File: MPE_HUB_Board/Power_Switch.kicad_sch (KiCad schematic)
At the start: 9 parts, among them U5 VND7050AJTR

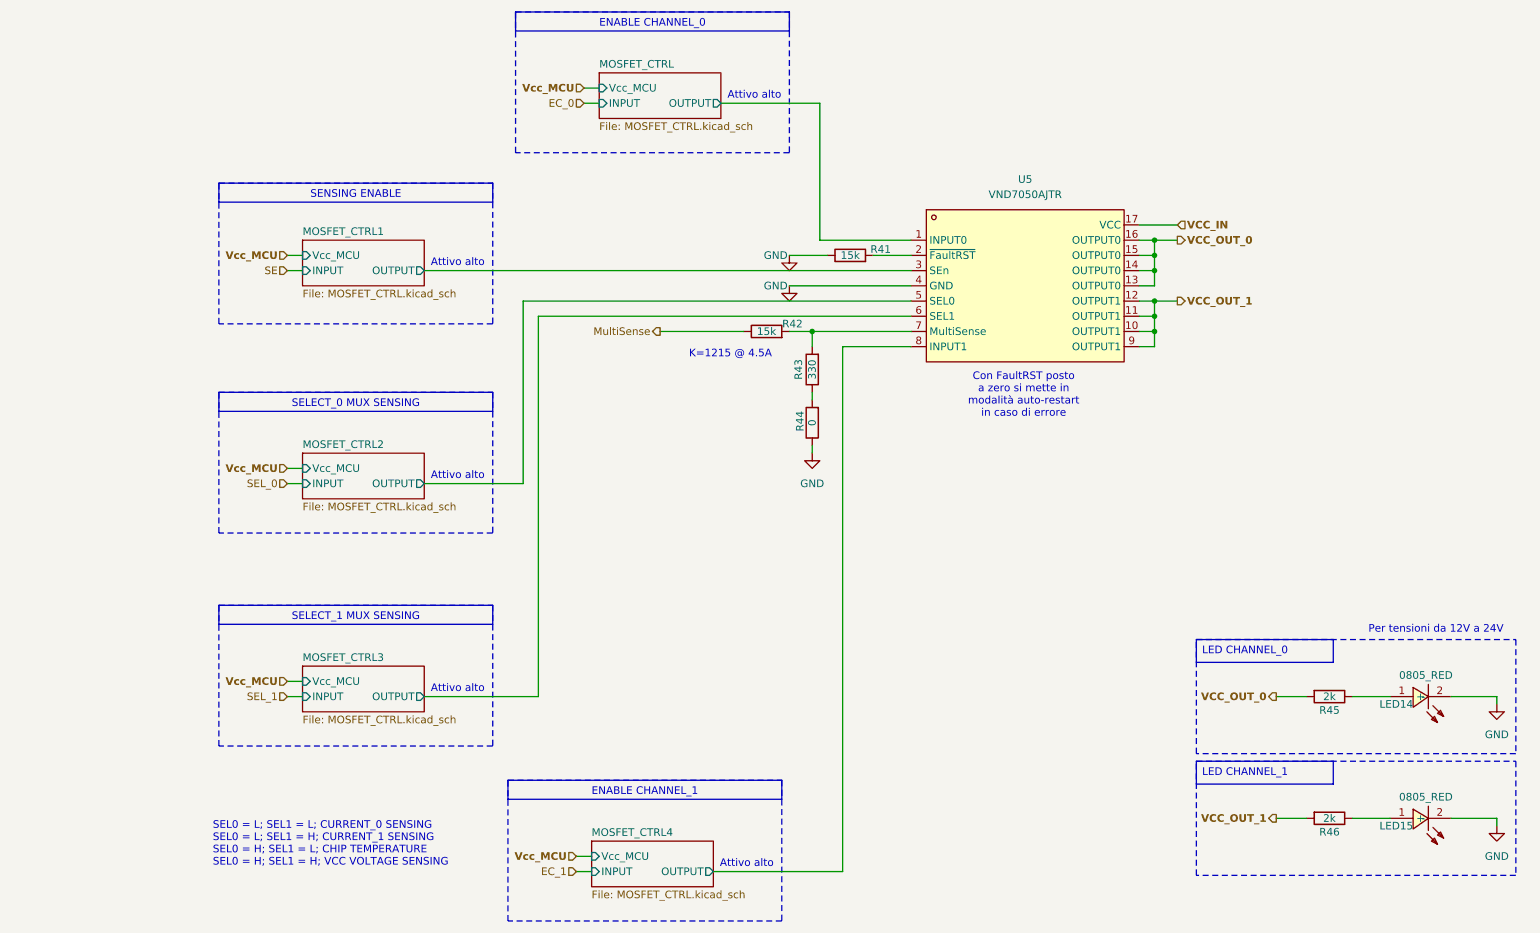
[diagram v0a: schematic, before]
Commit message: Update 04/07/2025
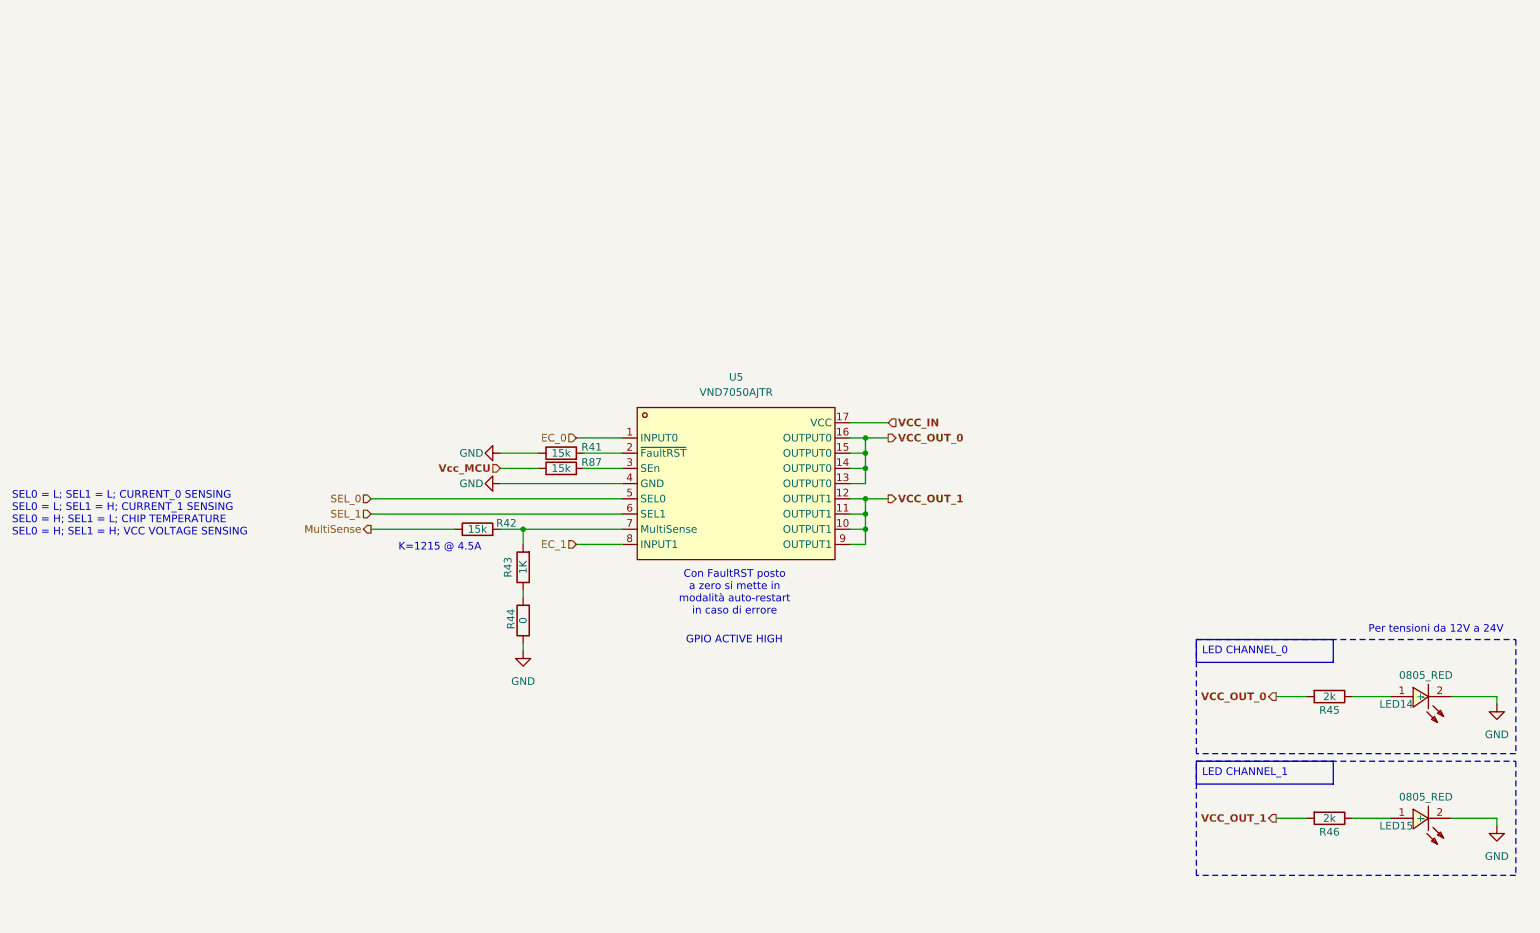
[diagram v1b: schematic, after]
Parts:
- added R87: 15k, Resistor_SMD:R_0603_1608Metric, symbol Device:R
- R43: value 330 -> 1K; LCSC C23138 -> C21190; LCSC Part (none) -> C21190
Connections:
- net MOSFET_CTRL/OUTPUT is gone; now on net EC_0: U5.1 (INPUT0)
- net MOSFET_CTRL2/OUTPUT is gone; now on net SEL_0: U5.5 (SEL0)
- net MOSFET_CTRL3/OUTPUT is gone; now on net SEL_1: U5.6 (SEL1)
- net MOSFET_CTRL4/OUTPUT is gone; now on net EC_1: U5.8 (INPUT1)
- net Vcc_MCU: now also R87.1
- net MOSFET_CTRL1/OUTPUT: no longer names the net of U5.3 (SEn)
- net MOSFET_CTRL1/OUTPUT: now also R87.2
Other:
- removed sheet MOSFET_CTRL
- removed sheet MOSFET_CTRL1
- removed sheet MOSFET_CTRL2
- removed sheet MOSFET_CTRL3
- removed sheet MOSFET_CTRL4
- note added: "GPIO ACTIVE HIGH"
- note removed: "Attivo alto"
- moved on the sheet: R41, R42, R44, U5

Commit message: Update 08/07/2025
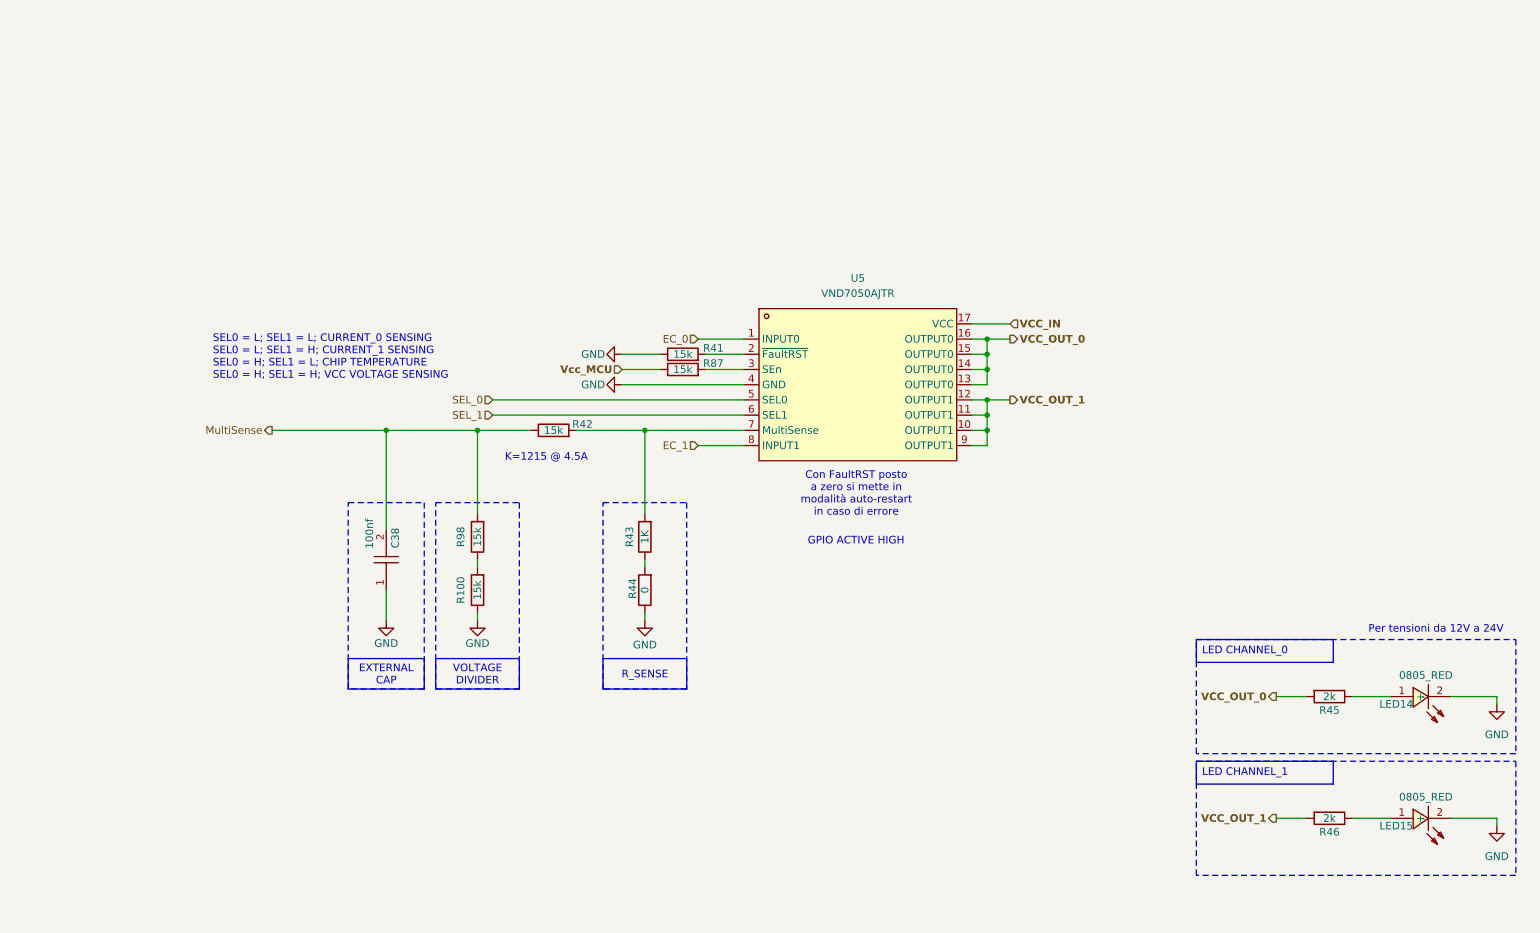
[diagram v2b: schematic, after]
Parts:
- added C38: 100nf, Capacitor_SMD:C_0603_1608Metric, symbol easyeda2kicad:CC0603KRX7R9BB104
- added R100, R98: 15k, Resistor_SMD:R_0603_1608Metric, symbol Device:R
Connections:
- net GND: now also C38.1, R100.1
- net MultiSense: now also C38.2, R98.2
- new net: R100.2, R98.1
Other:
- moved on the sheet: R41, R42, R43, R44, R87, U5

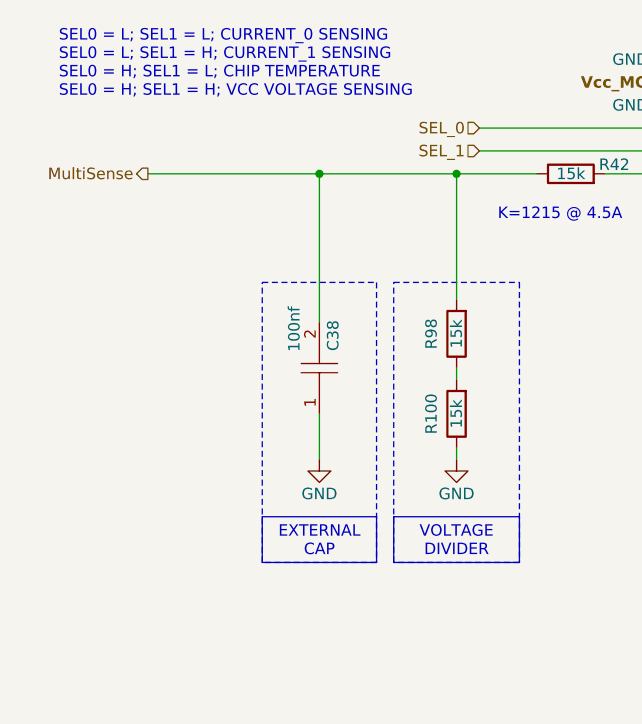
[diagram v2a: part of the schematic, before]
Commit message: HUB Hardware V1.1.0
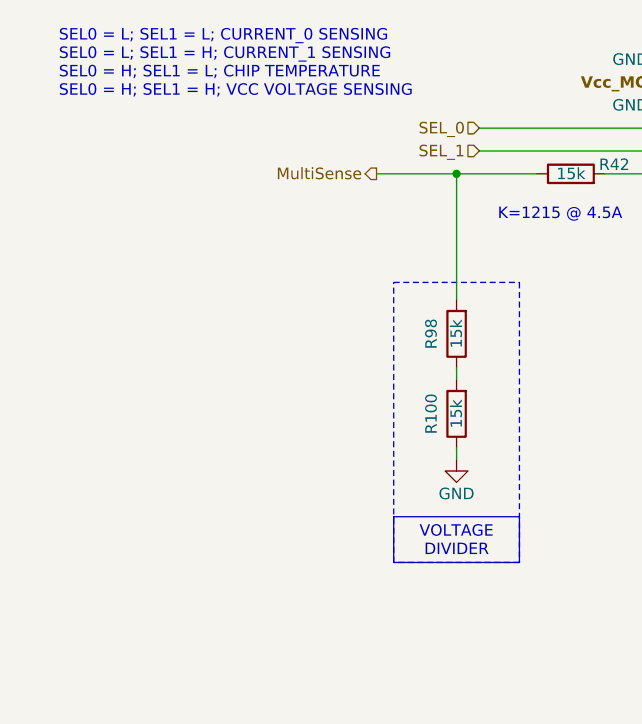
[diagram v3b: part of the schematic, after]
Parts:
- removed C38: 100nf, Capacitor_SMD:C_0603_1608Metric, symbol easyeda2kicad:CC0603KRX7R9BB104
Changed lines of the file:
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@@
-	)
-	(rectangle
-		(start 87.63 100.965)
-		(end 100.33 132.08)
-		(stroke
-			(width 0)
-			(type dot)
-			(color 0 132 0 1)
-		)
-		(fill
-			(type none)
-		)
 	)
 	(rectangle
@@
 		(at 102.235 127 0)
 		(size 13.97 5.08)
-		(margins 0.9525 0.9525 0.9525 0.9525)
-		(stroke
-			(width 0)
-			(type solid)
-			(color 0 132 0 1)
-		)
-		(fill
-			(type none)
-		)
-		(effects
-			(font
-				(size 1.27 1.27)
-				(color 0 132 0 1)
-			)
-		)
-	)
-	(text_box "EXTERNAL CAP"
-		(exclude_from_sim no)
-		(at 87.63 127 0)
-		(size 12.7 5.08)
 		(margins 0.9525 0.9525 0.9525 0.9525)
 		(stroke
@@
 	)
 	(junction
-		(at 93.98 88.9)
-		(diameter 0)
-		(color 0 0 0 0)
-	)
-	(junction
 		(at 194.31 78.74)
 		(diameter 0)
@@
 	(wire
 		(pts
-			(xy 93.98 115.57) (xy 93.98 120.65)
-		)
-		(stroke
-			(width 0)
-			(type default)
-		)
-	)
-	(wire
-		(pts
 			(xy 137.16 119.38) (xy 137.16 120.65)
 		)
@@
 	(wire
 		(pts
-			(xy 74.93 88.9) (xy 93.98 88.9)
-		)
-		(stroke
-			(width 0)
-			(type default)
-		)
-	)
-	(wire
-		(pts
-			(xy 93.98 88.9) (xy 93.98 105.41)
-		)
-		(stroke
-			(width 0)
-			(type default)
-		)
-	)
-	(wire
-		(pts
 			(xy 271.78 133.35) (xy 279.4 133.35)
 		)
@@
 	(wire
 		(pts
-			(xy 93.98 88.9) (xy 109.22 88.9)
+			(xy 100.33 88.9) (xy 109.22 88.9)
 		)
 		(stroke
@@
 	(hierarchical_label "MultiSense"
 		(shape output)
-		(at 74.93 88.9 180)
+		(at 100.33 88.9 180)
 		(effects
 			(font
@@
 				(path "/6490f62d-7c0a-4455-8633-837f094f0a1c/36a1afe1-9d7e-4453-8bd5-557c8a4303ef"
 					(reference "#PWR051")
-					(unit 1)
-				)
-			)
-		)
-	)
-	(symbol
-		(lib_name "CC0603KRX7R9BB104_2")
-		(lib_id "easyeda2kicad:CC0603KRX7R9BB104")
-		(at 93.98 110.49 90)
-		(unit 1)
-		(exclude_from_sim no)
-		(in_bom yes)
-		(on_board yes)
-		(dnp no)
-		(property "Reference" "C38"
-			(at 95.504 105.156 0)
-			(effects
-				(font
-					(size 1.27 1.27)
-				)
-				(justify right)
-			)
-		)
-		(property "Value" "100nf"
-			(at 91.186 103.632 0)
-			(effects
-				(font
-					(size 1.27 1.27)
-				)
-				(justify right)
-			)
-		)
-		(property "Footprint" "Capacitor_SMD:C_0603_1608Metric"
-			(at 101.6 110.49 0)
-			(effects
-				(font
-					(size 1.27 1.27)
-				)
-				(hide yes)
-			)
-		)
-		(property "Datasheet" "https://lcsc.com/product-detail/Multilayer-Ceramic-Capacitors-MLCC-SMD-SMT_100nF-104-10-50V_C14663.html"
-			(at 104.14 110.49 0)
-			(effects
-				(font
-					(size 1.27 1.27)
-				)
-				(hide yes)
-			)
-		)
-		(property "Description" ""
-			(at 93.98 110.49 0)
-			(effects
-				(font
-					(size 1.27 1.27)
-				)
-				(hide yes)
-			)
-		)
-		(property "LCSC Part" "C14663"
-			(at 106.68 110.49 0)
-			(effects
-				(font
-					(size 1.27 1.27)
-				)
-				(hide yes)
-			)
-		)
-		(property "LCSC" "C14663"
-			(at 95.885 107.95 0)
-			(effects
-				(font
-					(size 1.27 1.27)
-				)
-				(hide yes)
-			)
-		)
-		(pin "1"
-		)
-		(pin "2"
-		)
-		(instances
-			(project "HUB_MPE"
-				(path "/6490f62d-7c0a-4455-8633-837f094f0a1c/26b9dfe9-c957-43ca-ba2b-36e349e2ebb9"
-					(reference "C39")
-					(unit 1)
-				)
-				(path "/6490f62d-7c0a-4455-8633-837f094f0a1c/36a1afe1-9d7e-4453-8bd5-557c8a4303ef"
-					(reference "C38")
 					(unit 1)
 				)
@@
 					(unit 1)
 				)
-			)
-		)
-	)
-	(symbol
-		(lib_id "power:GND")
-		(at 93.98 120.65 0)
-		(unit 1)
-		(exclude_from_sim no)
-		(in_bom yes)
-		(on_board yes)
-		(dnp no)
-		(property "Reference" "#PWR083"
-			(at 93.98 127 0)
-			(effects
-				(font
-					(size 1.27 1.27)
-				)
-				(hide yes)
-			)
-		)
-		(property "Value" "GND"
-			(at 93.98 124.46 0)
-			(effects
-				(font
-					(size 1.27 1.27)
-				)
-			)
-		)
-		(property "Footprint" ""
-			(at 93.98 120.65 0)
-			(effects
-				(font
-					(size 1.27 1.27)
-				)
-				(hide yes)
-			)
-		)
-		(property "Datasheet" ""
-			(at 93.98 120.65 0)
-			(effects
-				(font
-					(size 1.27 1.27)
-				)
-				(hide yes)
-			)
-		)
-		(property "Description" "Power symbol creates a global label with name \"GND\" , ground"
-			(at 93.98 120.65 0)
-			(effects
-				(font
-					(size 1.27 1.27)
-				)
-				(hide yes)
-			)
-		)
-		(pin "1"
-		)
-		(instances
-			(project "HUB_MPE"
-				(path "/6490f62d-7c0a-4455-8633-837f094f0a1c/26b9dfe9-c957-43ca-ba2b-36e349e2ebb9"
-					(reference "#PWR084")
-					(unit 1)
-				)
-				(path "/6490f62d-7c0a-4455-8633-837f094f0a1c/36a1afe1-9d7e-4453-8bd5-557c8a4303ef"
-					(reference "#PWR083")
-					(unit 1)
-				)
